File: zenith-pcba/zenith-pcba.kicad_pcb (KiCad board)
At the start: 2 copper layers, 11 parts, among them SW1 G4R152312, U1 XC7A50T-CSG325, U2 K4B4G1646E-BCNB, U3 CH347T, X1 SX5B8.000F1520F30

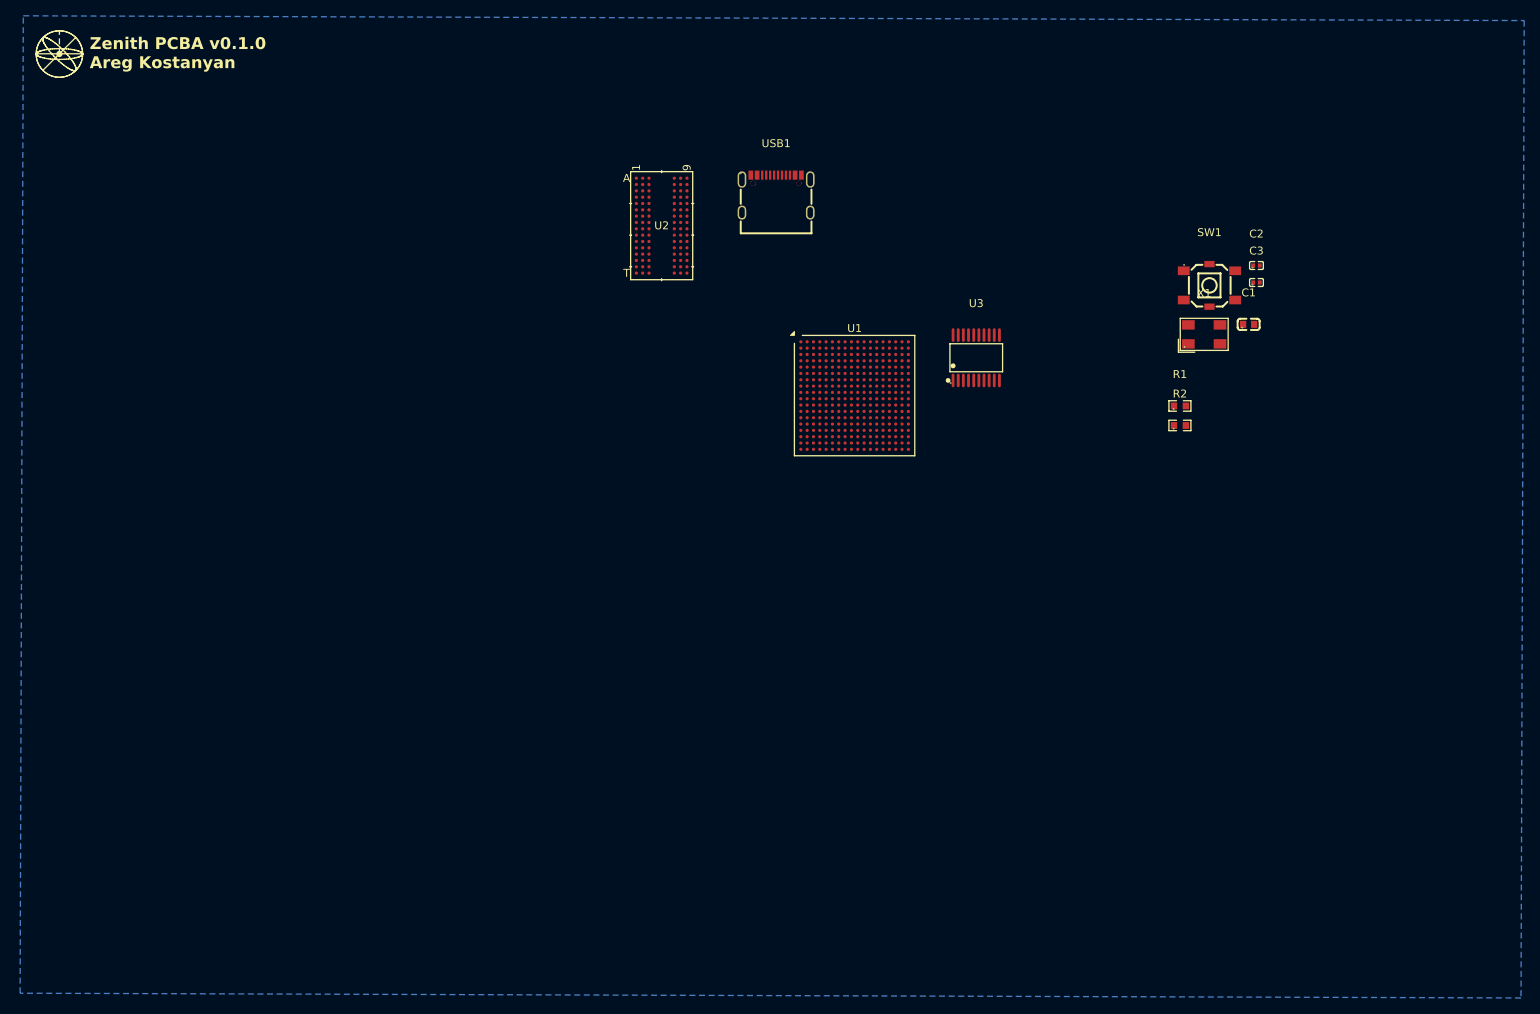
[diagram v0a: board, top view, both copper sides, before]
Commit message: fix(pcba): data routing
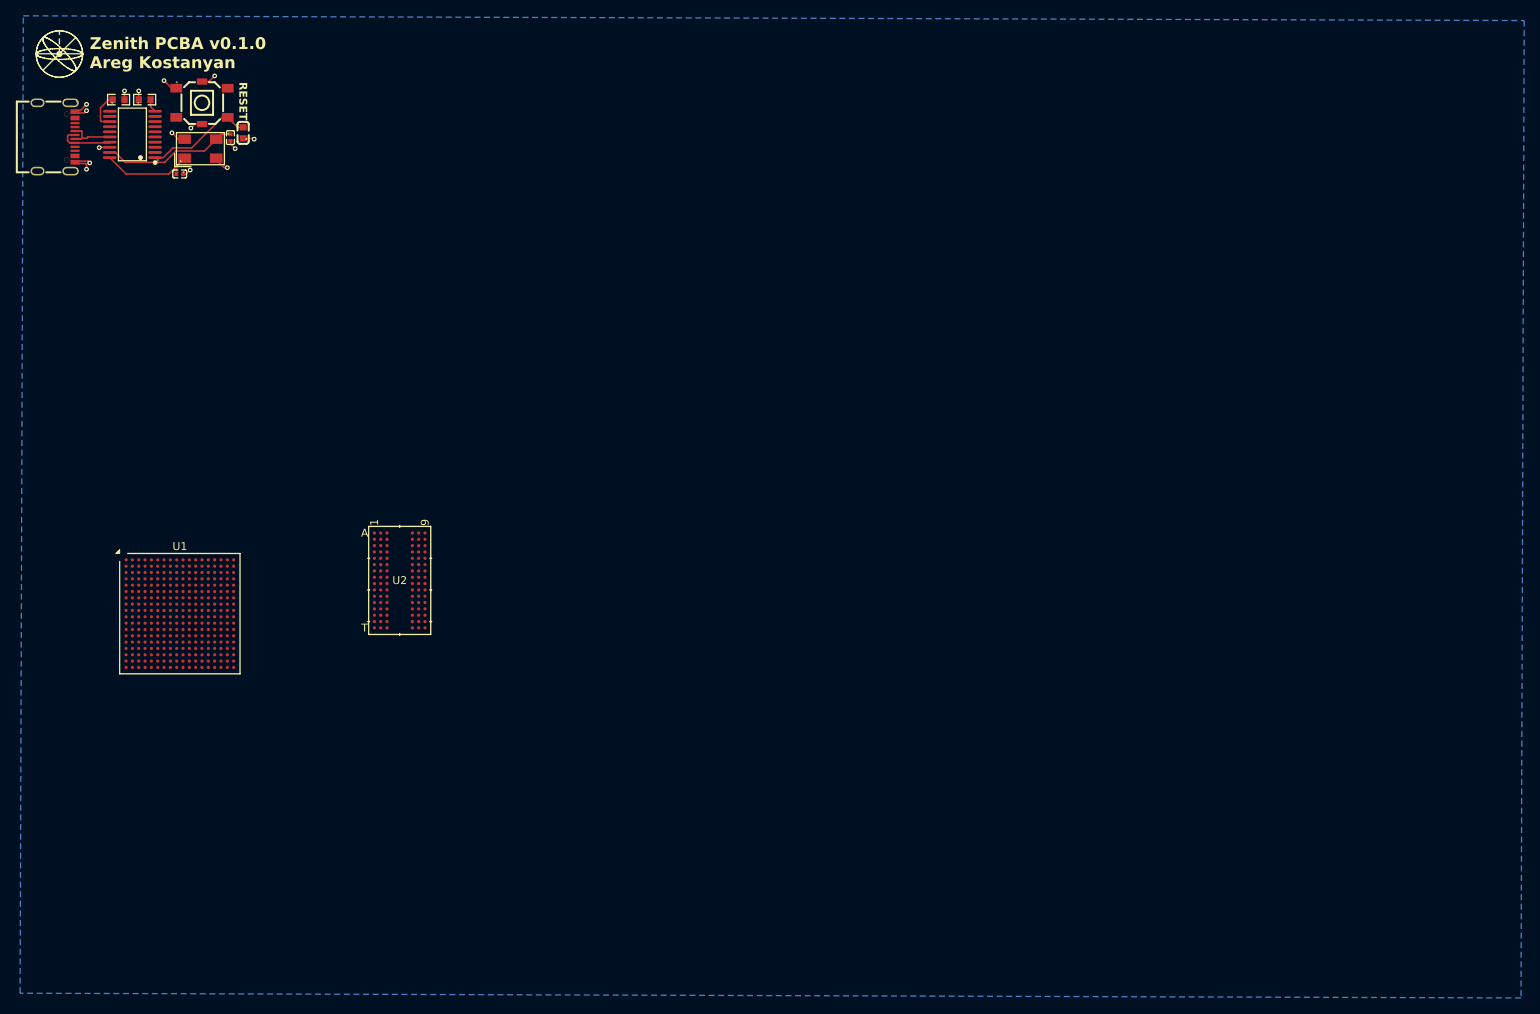
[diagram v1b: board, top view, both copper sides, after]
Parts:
- moved R2 140.4 mm to (69.5, 44.6)
- moved C2 136.7 mm to (77.2, 54.0), turned to 180 degrees
- moved R1 136.5 mm to (72.8, 44.6)
- moved C3 131.0 mm to (83.6, 49.4), turned to -90 degrees
- moved SW1 129.5 mm to (80.0, 45.0)
- moved C1 129.4 mm to (85.2, 48.8), turned to 90 degrees
- moved X1 129.1 mm to (79.8, 50.8)
- moved U3 110.4 mm to (71.2, 49.0), turned to 90 degrees
- moved USB1 91.3 mm to (61.6, 49.3), turned to -90 degrees
- moved U1 89.7 mm to (77.2, 109.6)
- moved U2 55.8 mm to (105.0, 105.4)
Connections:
- SW1 pad 5: unconnected-(SW1-NC-Pad5) -> GND
- SW1 pad 6: unconnected-(SW1-NC-Pad6) -> GND
- USB1 pad A1: unconnected-(USB1-GND-PadA1) -> GND
- USB1 pad A12: unconnected-(USB1-GND-PadA12) -> GND
- USB1 pad A6: unconnected-(USB1-DP1-PadA6) -> Net-(U3-UD+)
- USB1 pad A7: unconnected-(USB1-DN1-PadA7) -> Net-(U3-UD-)
- USB1 pad B1: unconnected-(USB1-GND-PadB1) -> GND
- USB1 pad B12: unconnected-(USB1-GND-PadB12) -> GND
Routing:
- net GND: track 0.00 -> 24.1 mm, vias 0 -> 15
- net Net-(U3-XI): track 0.00 -> 17.3 mm
- net Net-(U3-~{RST}): track 0.00 -> 13.8 mm
- net Net-(U3-XO): track 0.00 -> 12.1 mm
- net Net-(U3-UD+): track 0.00 -> 7.08 mm
- net Net-(U3-UD-): track 0.00 -> 6.25 mm
- net Net-(U3-RTS1/GPIO7): track 0.00 -> 4.81 mm
- net Net-(U3-TNOW1/DTR1): track 0.00 -> 1.71 mm
- added copper zone on B.Cu, net GND
- removed copper zone on B.Cu, net (none)
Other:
- board text added: "RESET"
